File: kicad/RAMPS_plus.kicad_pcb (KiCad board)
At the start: 2 copper layers, 122 x 68 mm, 134 parts, among them CON1 CON10, CON10 Stepstick_Left_Connector, CON11 Stepstick_Right_Connector, CON12 Stepstick_Left_Connector, CON13 Stepstick_Right_Connector, CON14 Stepstick_Left_Connector, CON15 Stepstick_Right_Connector, CON16 CON14x2, CON17 Stepstick_Left_Connector, CON18 Stepstick_Right_Connector, CON19 Stepstick_Left_Connector, CON2 CON8, CON20 Stepstick_Right_Connector, CON21 Panel1, CON22 Panel2, CON23 PS-ON, CON24 CON6, CON25 FAN, CON26 Chamber, CON27 BED, CON28 BED_Th, CON3 CON8, CON4 CON8, CON5 AUX, CON6 CON8, CON7 CON8, CON8 CON18x2, CON9 Carriage, Q1 IRLR2905ZPBF, Q2 IRLR2905ZPBF, Q3 FDC6401N, Q4 FDC6401N, Q5 IRLR2905ZPBF, Q6 FDC6401N, Q7 FDC6401N, Q8 FDC6401N, Q9 FDC6401N, SW1 RESET, U1 CD4504BPW, U2 SN74HCT245PW

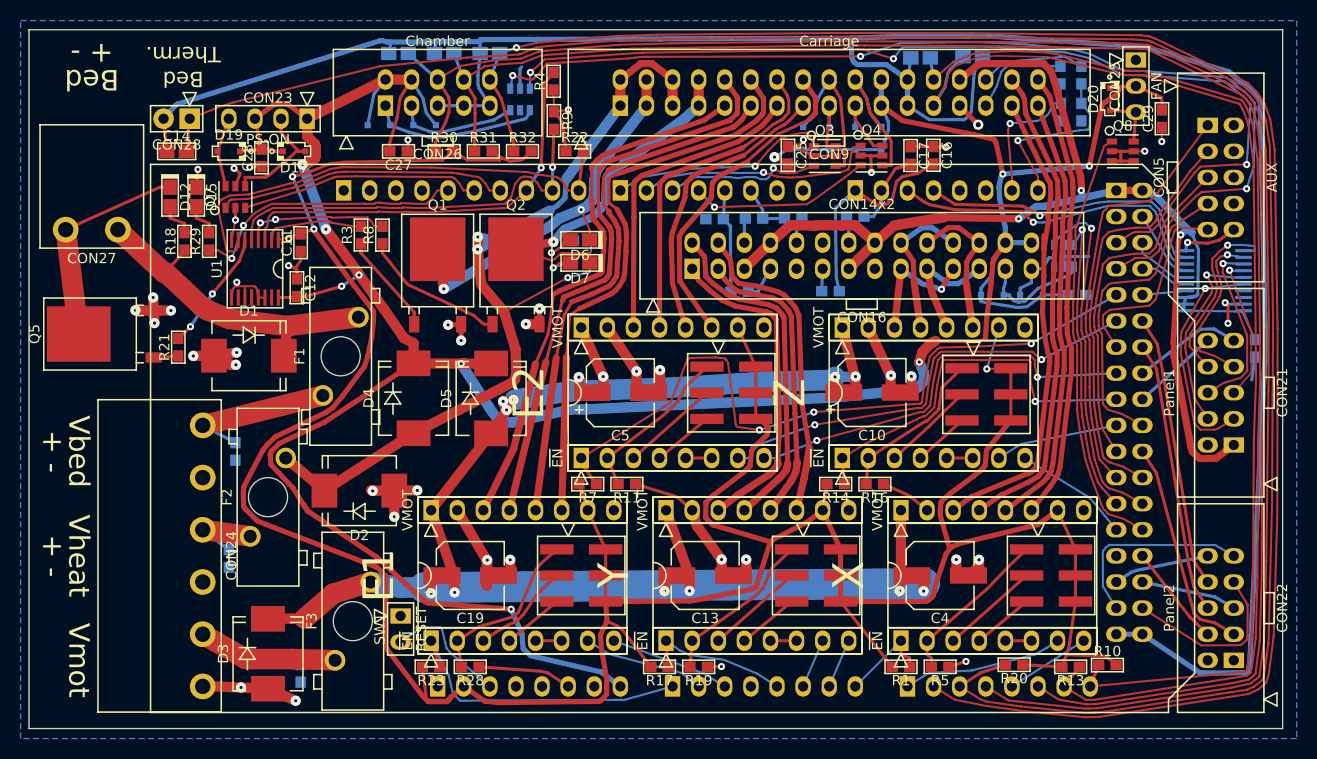
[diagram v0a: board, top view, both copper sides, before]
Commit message: Fix DRC issues.
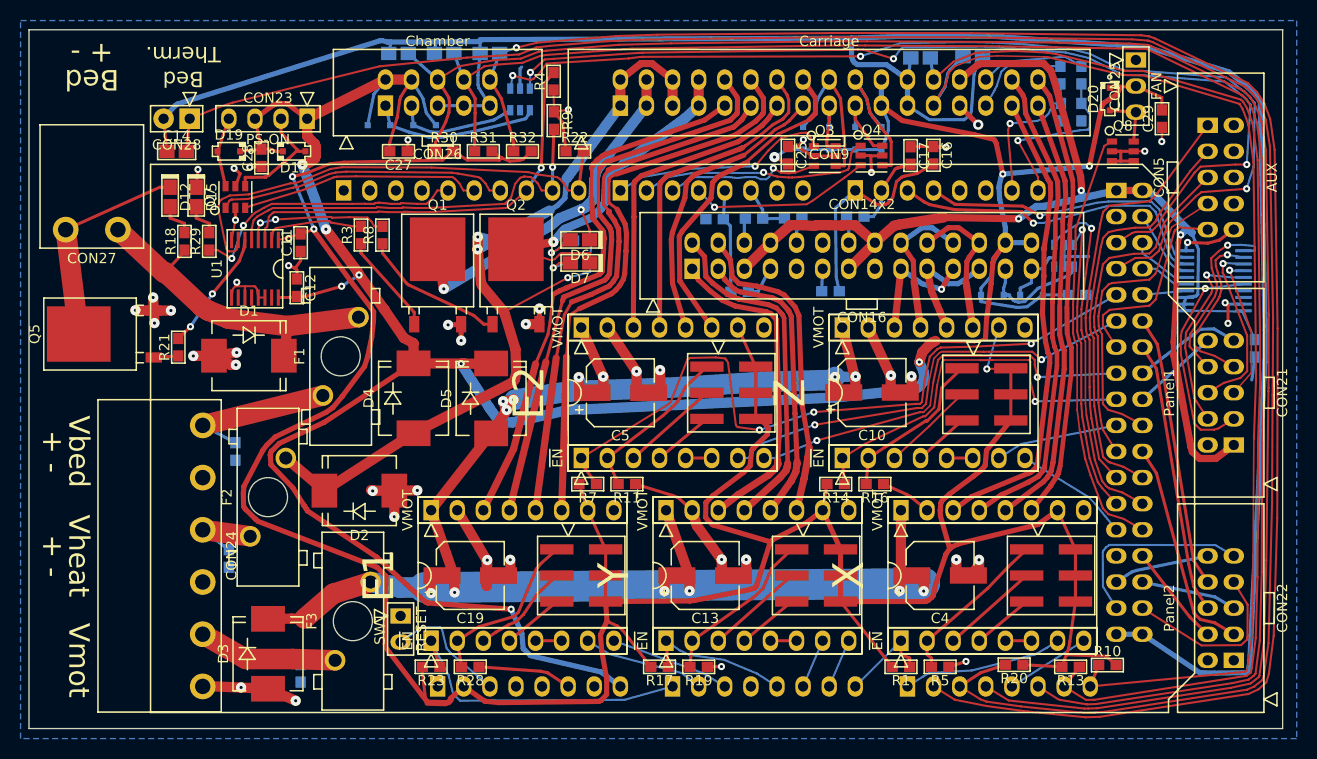
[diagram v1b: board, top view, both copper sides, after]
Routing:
- net /Carriage/XmotorA: track 46.8 -> 45.6 mm
